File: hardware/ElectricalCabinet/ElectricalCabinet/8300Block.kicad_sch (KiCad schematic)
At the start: 0 parts

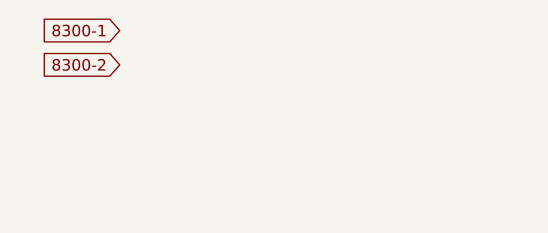
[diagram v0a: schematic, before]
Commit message: Electrical Cabinet done
Electrical Cabinet done, let me know if there are any changes or mistakes.
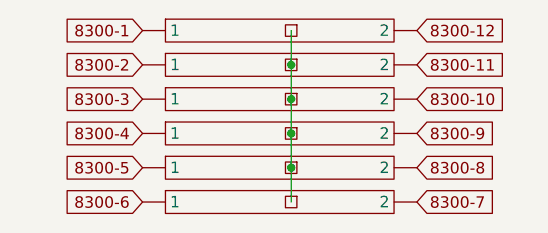
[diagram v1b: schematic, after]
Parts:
- added U64, U65, U66, U67, U68, U69: (no value), symbol TrafficLightLibrary:Terminal_Block
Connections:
- net 8300-1: now also U64. (2)
- net 8300-2: now also U65. (2)
- new net: U64. (2), U65. (2), U66. (2), U67. (2), U68. (2), U69. (2)
- new net 8300-10: U66. (2)
- new net 8300-11: U65. (2)
- new net 8300-12: U64. (2)
- new net 8300-3: U66. (2)
- new net 8300-4: U67. (2)
- new net 8300-5: U68. (2)
- new net 8300-6: U69. (2)
- new net 8300-7: U69. (2)
- new net 8300-8: U68. (2)
- new net 8300-9: U67. (2)
